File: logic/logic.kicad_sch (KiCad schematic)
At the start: 33 parts, among them J1 DIN41612_03x32_ABC, J2 Conn_02x05_Odd_Even, J3 Conn_02x05_Odd_Even, J4 Conn_02x05_Odd_Even, U1 TPIC6595, U2 TPIC6595, U3 TPIC6595, U4 TPIC6595, U5 TPIC6595, U6 TPIC6595, U7 TPIC6595, U8 TPIC6595, U9 74HC14

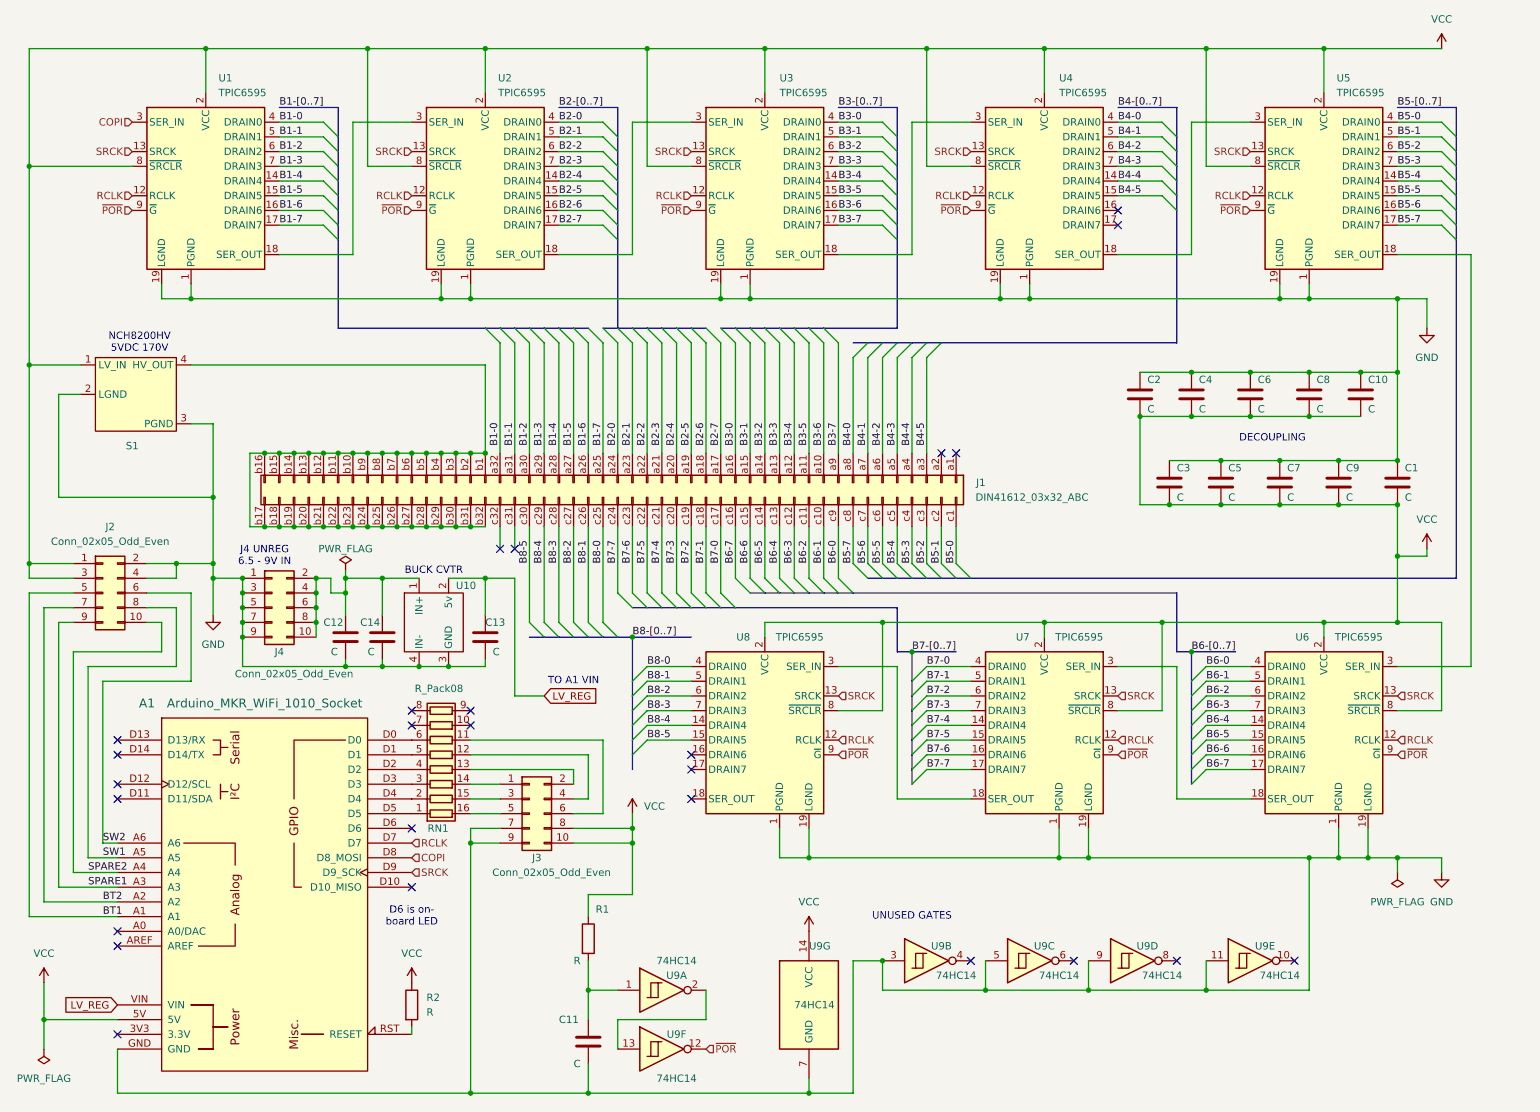
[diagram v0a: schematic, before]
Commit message: Begin incorporating feedback from prototype. Checkpoint.
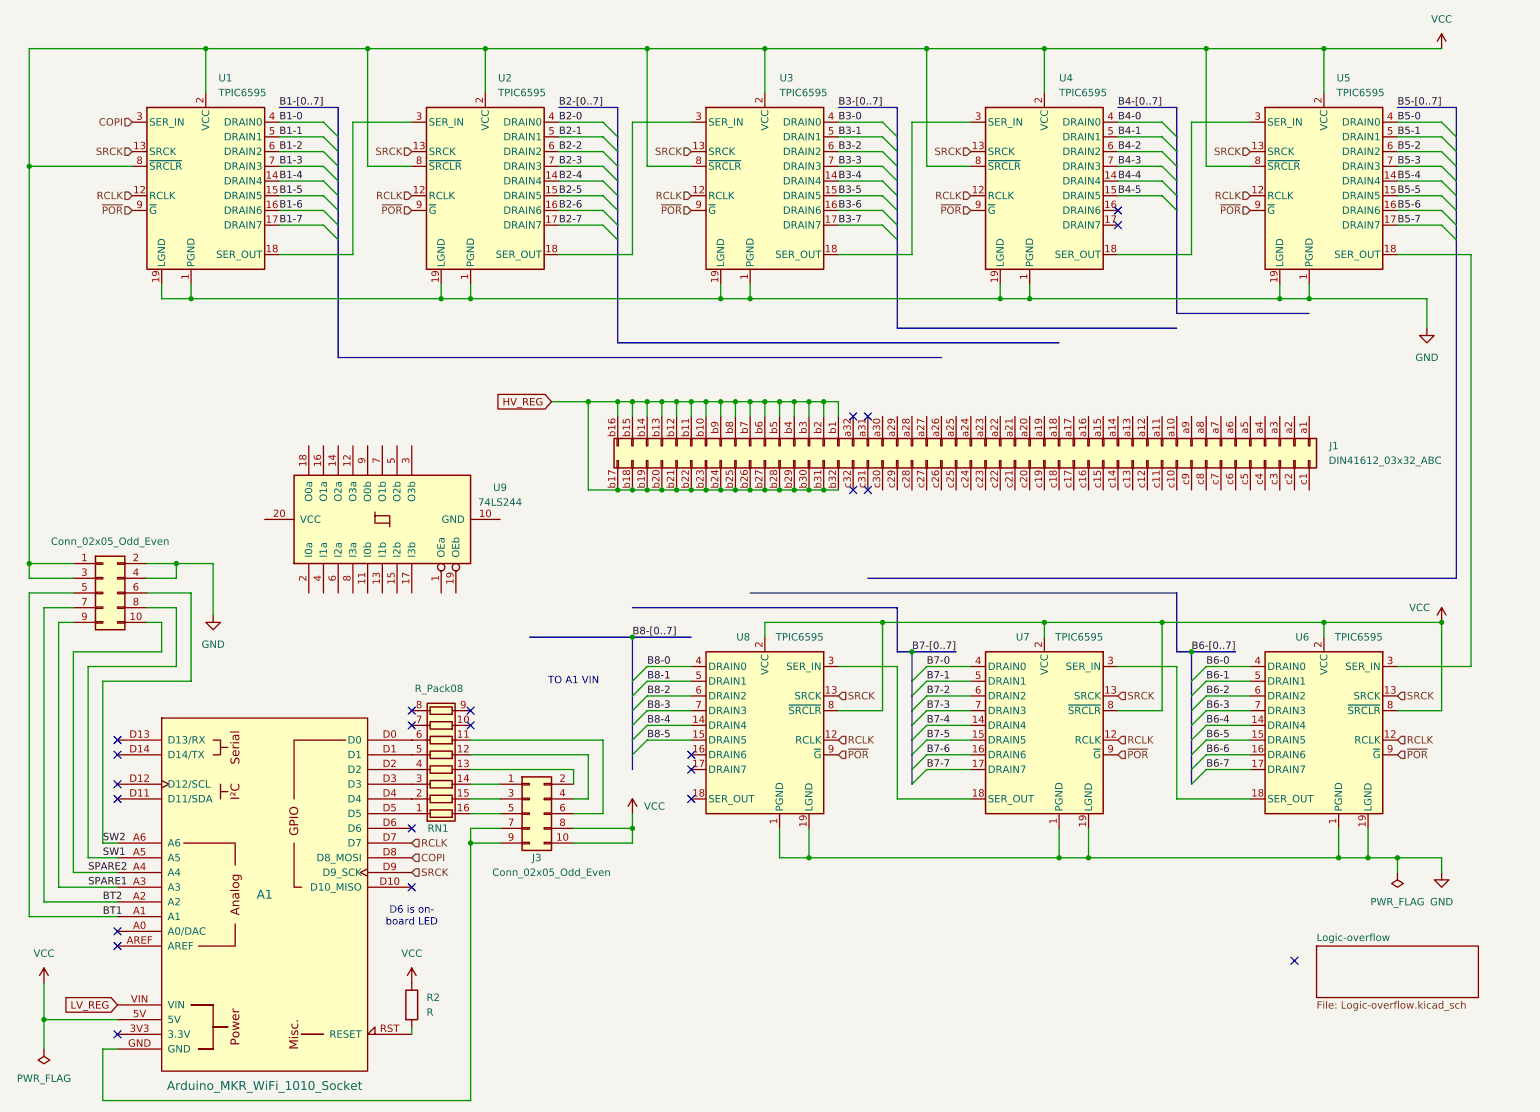
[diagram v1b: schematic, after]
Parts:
- removed C1, C10, C12, C13, C14, C2, C3, C4, C5, C6, C7, C8, C9: C, Capacitor_THT:C_Disc_D3.4mm_W2.1mm_P2.50mm, symbol Device:C
- removed C11: C, Capacitor_THT:CP_Radial_D8.0mm_P2.50mm, symbol Device:C
- removed J4: Conn_02x05_Odd_Even, Connector_PinHeader_2.54mm:PinHeader_2x05_P2.54mm_Vertical, symbol Connector_Generic:Conn_02x05_Odd_Even
- removed R1: R, Resistor_THT:R_Axial_DIN0207_L6.3mm_D2.5mm_P10.16mm_Horizontal, symbol Device:R
- removed S1: ~, NixComp:NCH8200HV, symbol NixComp:NCH8200HV_170v
- removed U10: ~, NixComp:TR4R7, symbol NixComp:TR4R7
- removed U9: 74HC14, Package_DIP:DIP-14_W7.62mm_Socket, symbol 74xx:74HC14
- added U9: 74LS244, symbol 74xx:74LS244
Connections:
- net B1-0: no longer J1.a32 (Pin_a32)
- net B1-1: no longer J1.a31 (Pin_a31)
- net B1-2: no longer J1.a30 (Pin_a30)
- net B1-3: no longer J1.a29 (Pin_a29)
- net B1-4: no longer J1.a28 (Pin_a28)
- net B1-5: no longer J1.a27 (Pin_a27)
- net B1-6: no longer J1.a26 (Pin_a26)
- net B1-7: no longer J1.a25 (Pin_a25)
- net B2-0: no longer J1.a24 (Pin_a24)
- net B2-1: no longer J1.a23 (Pin_a23)
- net B2-2: no longer J1.a22 (Pin_a22)
- net B2-3: no longer J1.a21 (Pin_a21)
- net B2-4: no longer J1.a20 (Pin_a20)
- net B2-5: no longer J1.a19 (Pin_a19)
- net B2-6: no longer J1.a18 (Pin_a18)
- net B2-7: no longer J1.a17 (Pin_a17)
- net B3-0: no longer J1.a16 (Pin_a16)
- net B3-1: no longer J1.a15 (Pin_a15)
- net B3-2: no longer J1.a14 (Pin_a14)
- net B3-3: no longer J1.a13 (Pin_a13)
- net B3-4: no longer J1.a12 (Pin_a12)
- net B3-5: no longer J1.a11 (Pin_a11)
- net B3-6: no longer J1.a10 (Pin_a10)
- net B3-7: no longer J1.a9 (Pin_a9)
- net B4-0: no longer J1.a8 (Pin_a8)
- net B4-1: no longer J1.a7 (Pin_a7)
- net B4-2: no longer J1.a6 (Pin_a6)
- net B4-3: no longer J1.a5 (Pin_a5)
- net B4-4: no longer J1.a4 (Pin_a4)
- net B4-5: no longer J1.a3 (Pin_a3)
- net B5-0: no longer J1.c1 (Pin_c1)
- net B5-1: no longer J1.c2 (Pin_c2)
- net B5-2: no longer J1.c3 (Pin_c3)
- net B5-3: no longer J1.c4 (Pin_c4)
- net B5-4: no longer J1.c5 (Pin_c5)
- net B5-5: no longer J1.c6 (Pin_c6)
- net B5-6: no longer J1.c7 (Pin_c7)
- net B5-7: no longer J1.c8 (Pin_c8)
- net B6-0: no longer J1.c9 (Pin_c9)
- net B6-1: no longer J1.c10 (Pin_c10)
- net B6-2: no longer J1.c11 (Pin_c11)
- net B6-3: no longer J1.c12 (Pin_c12)
- net B6-4: no longer J1.c13 (Pin_c13)
- net B6-5: no longer J1.c14 (Pin_c14)
- net B6-6: no longer J1.c15 (Pin_c15)
- net B6-7: no longer J1.c16 (Pin_c16)
- net B7-0: no longer J1.c17 (Pin_c17)
- net B7-1: no longer J1.c18 (Pin_c18)
- net B7-2: no longer J1.c19 (Pin_c19)
- net B7-3: no longer J1.c20 (Pin_c20)
- net B7-4: no longer J1.c21 (Pin_c21)
- net B7-5: no longer J1.c22 (Pin_c22)
- net B7-6: no longer J1.c23 (Pin_c23)
- net B7-7: no longer J1.c24 (Pin_c24)
- net B8-0: no longer J1.c25 (Pin_c25)
- net B8-1: no longer J1.c26 (Pin_c26)
- net B8-2: no longer J1.c27 (Pin_c27)
- net B8-3: no longer J1.c28 (Pin_c28)
- net B8-4: no longer J1.c29 (Pin_c29)
- net B8-5: no longer J1.c30 (Pin_c30)
- net GND: no longer A1.GND, J3.7 (Pin_7), J3.9 (Pin_9)
- net HV_REG: now reaches J1.b1 (Pin_b1), J1.b10 (Pin_b10), J1.b11 (Pin_b11), J1.b12 (Pin_b12), J1.b13 (Pin_b13), J1.b14 (Pin_b14), J1.b15 (Pin_b15), J1.b16 (Pin_b16), J1.b17 (Pin_b17), J1.b18 (Pin_b18), J1.b19 (Pin_b19), J1.b2 (Pin_b2), J1.b20 (Pin_b20), J1.b21 (Pin_b21), J1.b22 (Pin_b22), J1.b23 (Pin_b23), J1.b24 (Pin_b24), J1.b25 (Pin_b25), J1.b26 (Pin_b26), J1.b27 (Pin_b27), J1.b28 (Pin_b28), J1.b29 (Pin_b29), J1.b3 (Pin_b3), J1.b30 (Pin_b30), J1.b31 (Pin_b31), J1.b32 (Pin_b32), J1.b4 (Pin_b4), J1.b5 (Pin_b5), J1.b6 (Pin_b6), J1.b7 (Pin_b7), J1.b8 (Pin_b8), J1.b9 (Pin_b9)
- new net: A1.GND, J3.7 (Pin_7), J3.9 (Pin_9)
- no-connect marks 26 -> 23
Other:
- added sheet Logic-overflow (Logic-overflow.kicad_sch)
- note removed: "BUCK CVTR"
- note removed: "DECOUPLING"
- note removed: "J4 UNREG 6.5 - 9V IN"
- note removed: "NCH8200HV 5VDC 170V"
- note removed: "UNUSED GATES"
- moved on the sheet: J1
